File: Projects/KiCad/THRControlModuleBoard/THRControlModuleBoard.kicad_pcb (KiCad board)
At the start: 2 copper layers, 81.8 x 76.2 mm, 24 parts, among them J3 Screw_Terminal_01x02, Q1 Q_PMOS_GDS, Q2 Q_PMOS_GDS, Q3 Q_PMOS_GDS, U1 LTC4416EMS#PBF, U2 MAX31856MUD+T

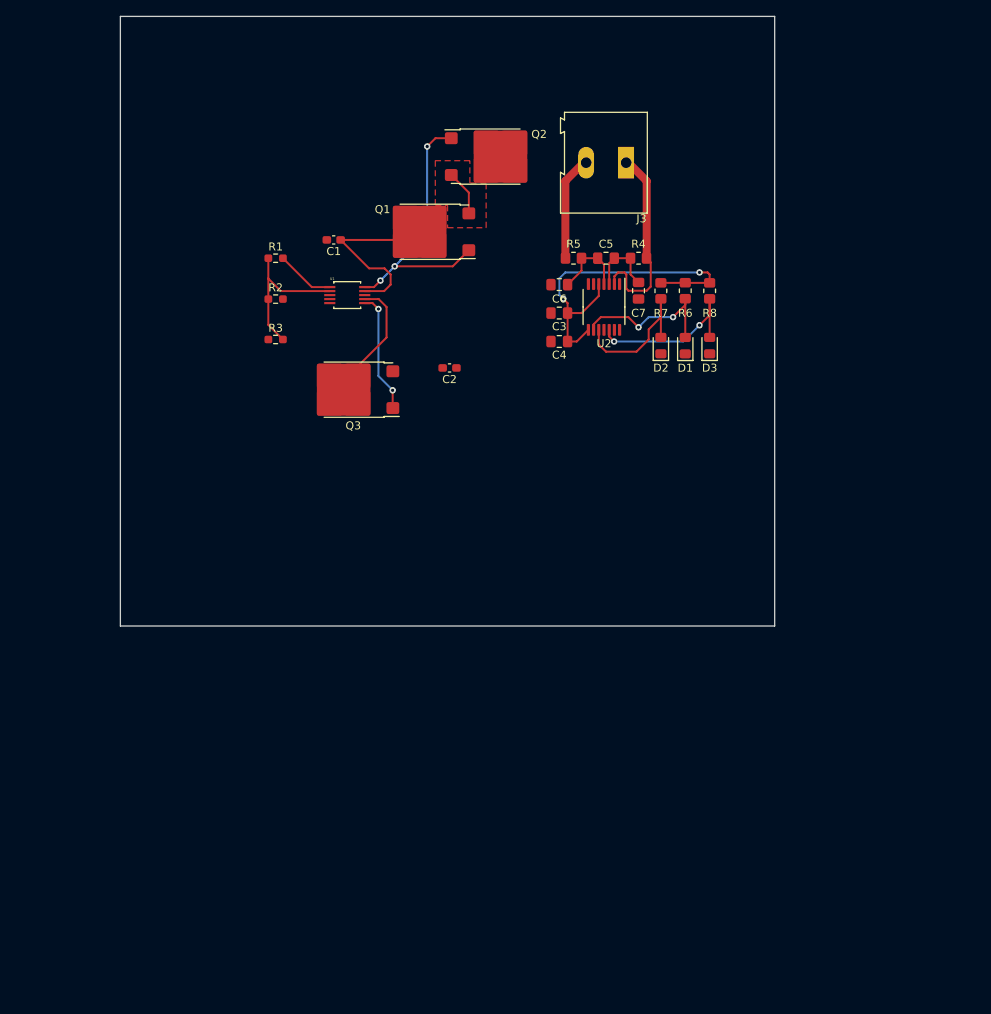
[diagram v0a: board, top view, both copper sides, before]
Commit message: THRControlModuleBoardを更新
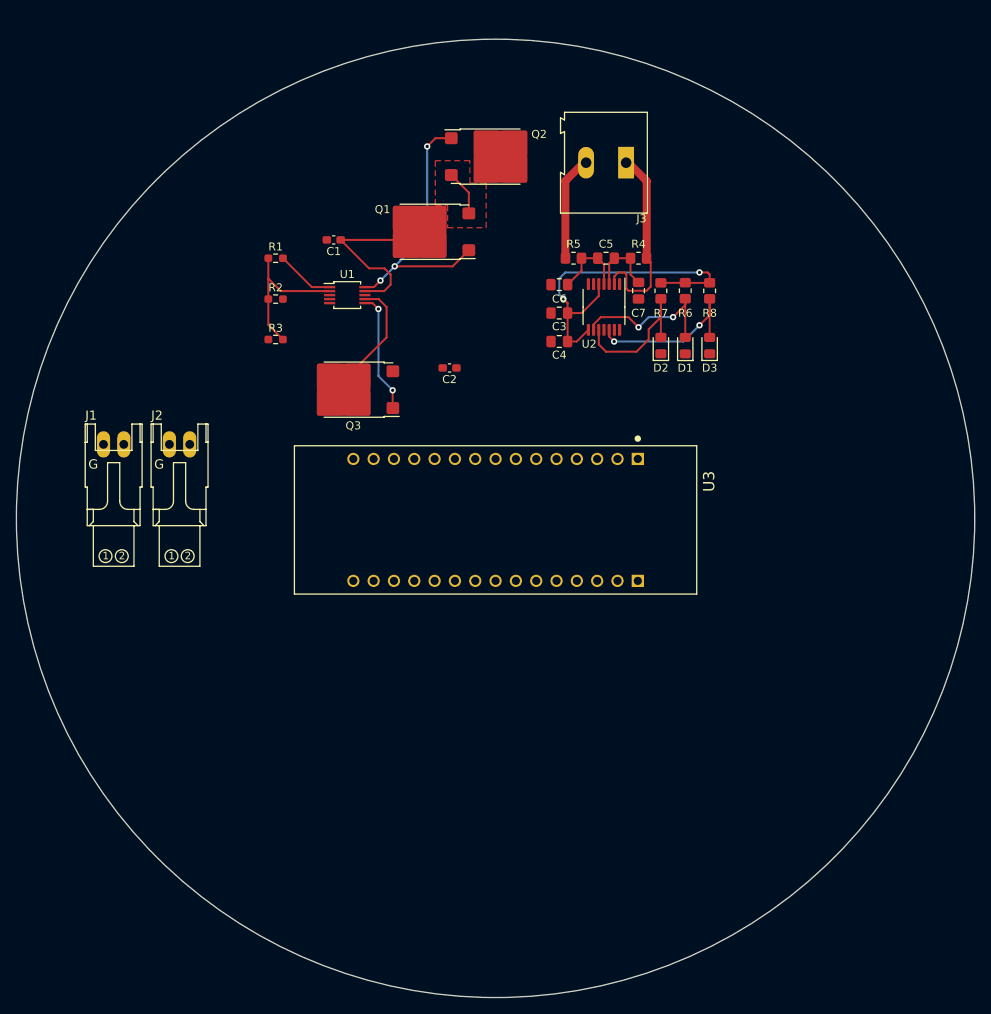
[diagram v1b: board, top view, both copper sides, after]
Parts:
- added J1: Conn_01x02_Socket, CONNECTOR:CONNECTOR_2, F.Cu at (126.2, 108.4)
- added J2: Conn_01x02_Socket, CONNECTOR:CONNECTOR_2, F.Cu at (134.4, 108.4)
- added U3: NUCLEO-F303K8, NUCLEO-F303K8:MODULE_NUCLEO-F303K8, F.Cu at (173.9, 114.0)
- U1: footprint LTC4416EMS#PBF:MSOP-10_MS -> Package_SO:MSOP-10_3x3mm_P0.5mm
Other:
- board size 81.8 x 76.2 mm -> 119.8 x 119.8 mm
